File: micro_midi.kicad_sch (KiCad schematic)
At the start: 67 parts, among them U1 74HC595, U2 Arduino_Micro, U3 74HC595

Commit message: resistor change and pdf
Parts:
- R1, R10, R11, R12, R13, R14, R15, R16, R2, R3, R4, R5, R6, R7, R8, R9: footprint ScottoKeebs_Components:Resistor_0402 -> Resistor_THT:R_Axial_DIN0204_L3.6mm_D1.6mm_P1.90mm_Vertical
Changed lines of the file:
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@@
 			)
 		)
-		(property "Footprint" "ScottoKeebs_Components:Resistor_0402"
+		(property "Footprint" "Resistor_THT:R_Axial_DIN0204_L3.6mm_D1.6mm_P1.90mm_Vertical"
 			(at 218.44 124.968 0)
 			(effects
@@
 			)
 		)
-		(property "Footprint" "ScottoKeebs_Components:Resistor_0402"
+		(property "Footprint" "Resistor_THT:R_Axial_DIN0204_L3.6mm_D1.6mm_P1.90mm_Vertical"
 			(at 218.44 114.808 0)
 			(effects
@@
 			)
 		)
-		(property "Footprint" "ScottoKeebs_Components:Resistor_0402"
+		(property "Footprint" "Resistor_THT:R_Axial_DIN0204_L3.6mm_D1.6mm_P1.90mm_Vertical"
 			(at 218.44 112.268 0)
 			(effects
@@
 			)
 		)
-		(property "Footprint" "ScottoKeebs_Components:Resistor_0402"
+		(property "Footprint" "Resistor_THT:R_Axial_DIN0204_L3.6mm_D1.6mm_P1.90mm_Vertical"
 			(at 218.44 117.348 0)
 			(effects
@@
 			)
 		)
-		(property "Footprint" "ScottoKeebs_Components:Resistor_0402"
+		(property "Footprint" "Resistor_THT:R_Axial_DIN0204_L3.6mm_D1.6mm_P1.90mm_Vertical"
 			(at 218.44 66.548 0)
 			(effects
@@
 			)
 		)
-		(property "Footprint" "ScottoKeebs_Components:Resistor_0402"
+		(property "Footprint" "Resistor_THT:R_Axial_DIN0204_L3.6mm_D1.6mm_P1.90mm_Vertical"
 			(at 218.44 71.628 0)
 			(effects
@@
 			)
 		)
-		(property "Footprint" "ScottoKeebs_Components:Resistor_0402"
+		(property "Footprint" "Resistor_THT:R_Axial_DIN0204_L3.6mm_D1.6mm_P1.90mm_Vertical"
 			(at 218.44 109.728 0)
 			(effects
@@
 			)
 		)
-		(property "Footprint" "ScottoKeebs_Components:Resistor_0402"
+		(property "Footprint" "Resistor_THT:R_Axial_DIN0204_L3.6mm_D1.6mm_P1.90mm_Vertical"
 			(at 218.44 58.928 0)
 			(effects
@@
 			)
 		)
-		(property "Footprint" "ScottoKeebs_Components:Resistor_0402"
+		(property "Footprint" "Resistor_THT:R_Axial_DIN0204_L3.6mm_D1.6mm_P1.90mm_Vertical"
 			(at 218.44 64.008 0)
 			(effects
@@
 			)
 		)
-		(property "Footprint" "ScottoKeebs_Components:Resistor_0402"
+		(property "Footprint" "Resistor_THT:R_Axial_DIN0204_L3.6mm_D1.6mm_P1.90mm_Vertical"
 			(at 218.44 107.188 0)
 			(effects
@@
 			)
 		)
-		(property "Footprint" "ScottoKeebs_Components:Resistor_0402"
+		(property "Footprint" "Resistor_THT:R_Axial_DIN0204_L3.6mm_D1.6mm_P1.90mm_Vertical"
 			(at 218.44 61.468 0)
 			(effects
@@
 			)
 		)
-		(property "Footprint" "ScottoKeebs_Components:Resistor_0402"
+		(property "Footprint" "Resistor_THT:R_Axial_DIN0204_L3.6mm_D1.6mm_P1.90mm_Vertical"
 			(at 218.44 122.428 0)
 			(effects
@@
 			)
 		)
-		(property "Footprint" "ScottoKeebs_Components:Resistor_0402"
+		(property "Footprint" "Resistor_THT:R_Axial_DIN0204_L3.6mm_D1.6mm_P1.90mm_Vertical"
 			(at 218.44 69.088 0)
 			(effects
@@
 			)
 		)
-		(property "Footprint" "ScottoKeebs_Components:Resistor_0402"
+		(property "Footprint" "Resistor_THT:R_Axial_DIN0204_L3.6mm_D1.6mm_P1.90mm_Vertical"
 			(at 218.44 56.388 0)
 			(effects
@@
 			)
 		)
-		(property "Footprint" "ScottoKeebs_Components:Resistor_0402"
+		(property "Footprint" "Resistor_THT:R_Axial_DIN0204_L3.6mm_D1.6mm_P1.90mm_Vertical"
 			(at 218.44 119.888 0)
 			(effects
@@
 			)
 		)
-		(property "Footprint" "ScottoKeebs_Components:Resistor_0402"
+		(property "Footprint" "Resistor_THT:R_Axial_DIN0204_L3.6mm_D1.6mm_P1.90mm_Vertical"
 			(at 218.44 74.168 0)
 			(effects

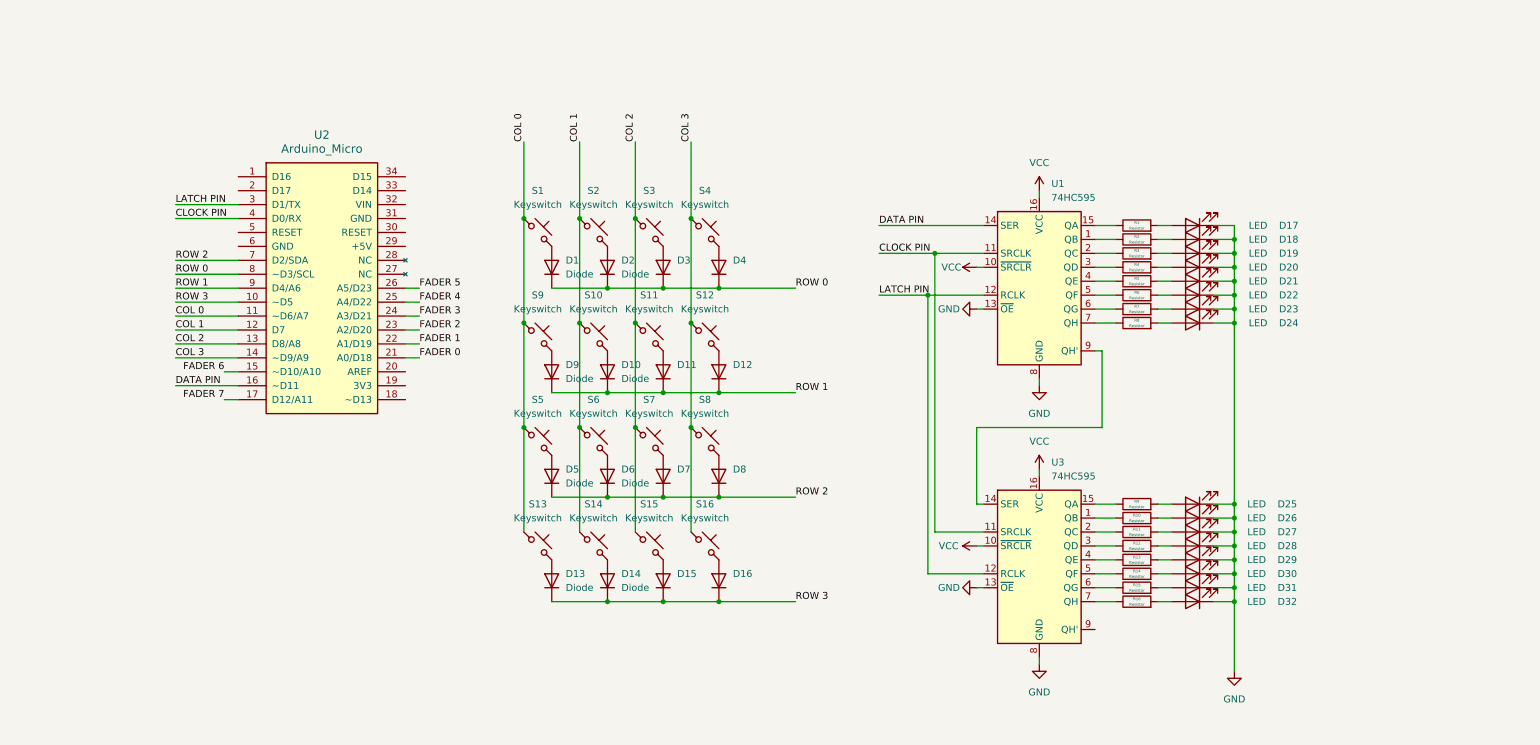
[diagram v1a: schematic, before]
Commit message: nearing completion
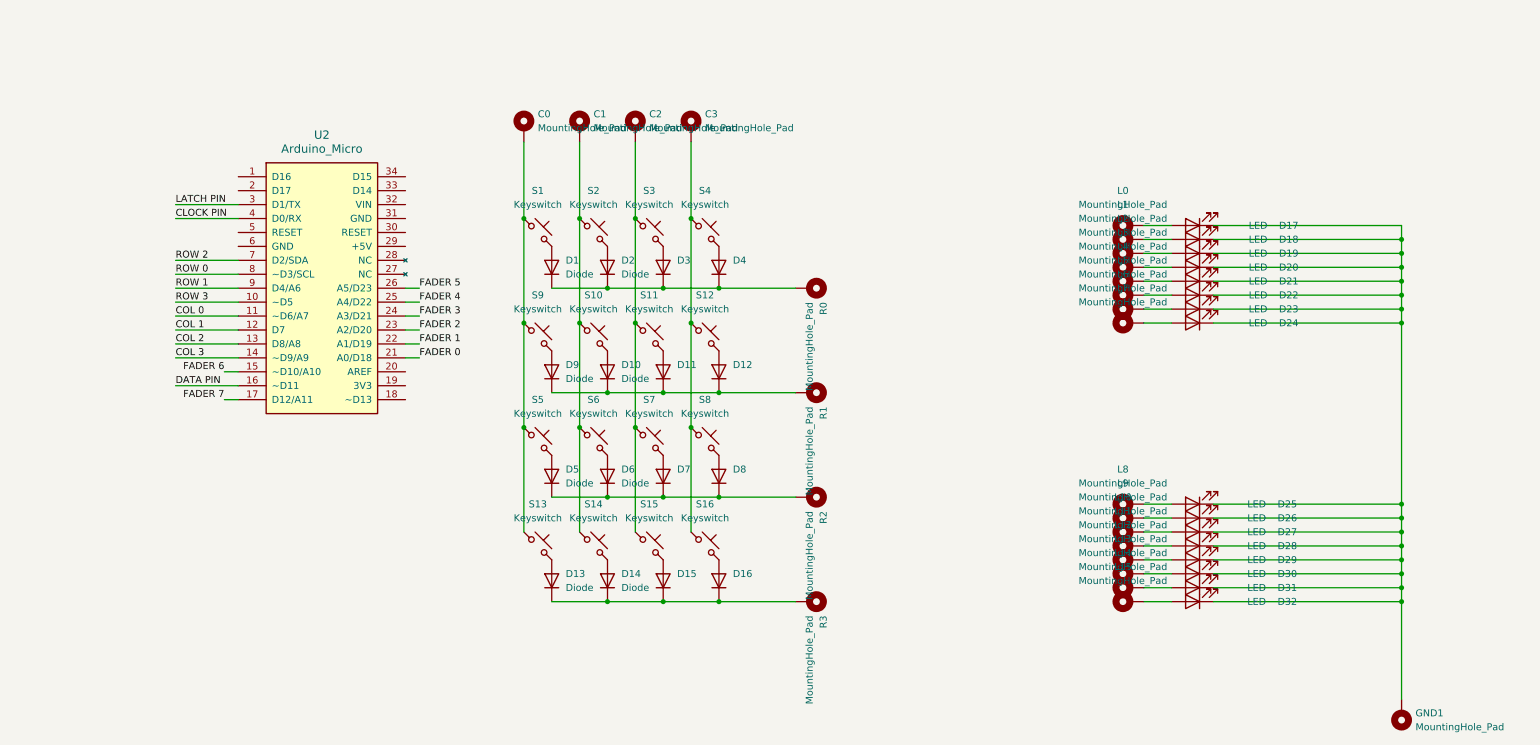
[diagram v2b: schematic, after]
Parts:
- removed R1, R10, R11, R12, R13, R14, R15, R16, R2, R3, R4, R5, R6, R7, R8, R9: Resistor, Resistor_THT:R_Axial_DIN0204_L3.6mm_D1.6mm_P1.90mm_Vertical, symbol ScottoKeebs:Placeholder_Resistor
- removed U1, U3: 74HC595, Package_SO:SSOP-16_5.3x6.2mm_P0.65mm, symbol 74xx:74HC595
- added C0, C1, C2, C3, GND1, L0, L1, L10, L11, L12, L13, L14, L15, L2, L3, L4, L5, L6, L7, L8, L9, R0, R1, R2, R3: MountingHole_Pad, TestPoint:TestPoint_Plated_Hole_D3.0mm, symbol Mechanical:MountingHole_Pad
- U2: footprint Arduino:Arduino_Micro -> (none)
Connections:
- net COL 0: no longer S1.1, S13.1, S5.1, S9.1
- net COL 1: no longer S10.1, S14.1, S2.1, S6.1
- net COL 2: no longer S11.1, S15.1, S3.1, S7.1
- net COL 3: no longer S12.1, S16.1, S4.1, S8.1
- net ROW 0: no longer D1.1 (K), D2.1 (K), D3.1 (K), D4.1 (K)
- net ROW 1: no longer D10.1 (K), D11.1 (K), D12.1 (K), D9.1 (K)
- net ROW 2: no longer D5.1 (K), D6.1 (K), D7.1 (K), D8.1 (K)
- net ROW 3: no longer D13.1 (K), D14.1 (K), D15.1 (K), D16.1 (K)
- net at D24.2 (A): now also L7.1
- net at D32.2 (A): now also L15.1
- net at D31.2 (A): now also L14.1
- net at D26.2 (A): now also L9.1
- net at D23.2 (A): now also L6.1
- net at D22.2 (A): now also L5.1
- net at D28.2 (A): now also L11.1
- net at D27.2 (A): now also L10.1
- net at D29.2 (A): now also L12.1
- net at D21.2 (A): now also L4.1
- net at D25.2 (A): now also L8.1
- net at D17.2 (A): now also L0.1
- net at D18.2 (A): now also L1.1
- net at D30.2 (A): now also L13.1
- net at D20.2 (A): now also L3.1
- net at D19.2 (A): now also L2.1
- net GND: no longer names the net of D17.1 (K), D18.1 (K), D19.1 (K), D20.1 (K), D21.1 (K), D22.1 (K), D23.1 (K), D24.1 (K), D25.1 (K), D26.1 (K), D27.1 (K), D28.1 (K), D29.1 (K), D30.1 (K), D31.1 (K), D32.1 (K)
- net GND: now also GND1.1
- new net: D10.1 (K), D11.1 (K), D12.1 (K), D9.1 (K), R1.1
- new net: C1.1, S10.1, S14.1, S2.1, S6.1
- new net: D13.1 (K), D14.1 (K), D15.1 (K), D16.1 (K), R3.1
- new net: D5.1 (K), D6.1 (K), D7.1 (K), D8.1 (K), R2.1
- new net: D1.1 (K), D2.1 (K), D3.1 (K), D4.1 (K), R0.1
- new net: C3.1, S12.1, S16.1, S4.1, S8.1
- new net: C0.1, S1.1, S13.1, S5.1, S9.1
- new net: C2.1, S11.1, S15.1, S3.1, S7.1

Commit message: updates
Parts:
- C0, C1, C2, C3, GND1, L0, L1, L10, L11, L12, L13, L14, L15, L2, L3, L4, L5, L6, L7, L8, L9, R0, R1, R2, R3: footprint TestPoint:TestPoint_Plated_Hole_D3.0mm -> CustomLib:THROUGH HOLE PAD 1.7MM HOLE 3.0MM PAD
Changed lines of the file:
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@@
 			)
 		)
-		(property "Footprint" "TestPoint:TestPoint_Plated_Hole_D3.0mm"
+		(property "Footprint" "CustomLib:THROUGH HOLE PAD 1.7MM HOLE 3.0MM PAD"
 			(at 158.75 85.09 0)
 			(effects
@@
 			)
 		)
-		(property "Footprint" "TestPoint:TestPoint_Plated_Hole_D3.0mm"
+		(property "Footprint" "CustomLib:THROUGH HOLE PAD 1.7MM HOLE 3.0MM PAD"
 			(at 116.84 36.83 0)
 			(effects
@@
 			)
 		)
-		(property "Footprint" "TestPoint:TestPoint_Plated_Hole_D3.0mm"
+		(property "Footprint" "CustomLib:THROUGH HOLE PAD 1.7MM HOLE 3.0MM PAD"
 			(at 217.17 120.65 0)
 			(effects
@@
 			)
 		)
-		(property "Footprint" "TestPoint:TestPoint_Plated_Hole_D3.0mm"
+		(property "Footprint" "CustomLib:THROUGH HOLE PAD 1.7MM HOLE 3.0MM PAD"
 			(at 266.7 143.51 0)
 			(effects
@@
 			)
 		)
-		(property "Footprint" "TestPoint:TestPoint_Plated_Hole_D3.0mm"
+		(property "Footprint" "CustomLib:THROUGH HOLE PAD 1.7MM HOLE 3.0MM PAD"
 			(at 217.17 113.03 0)
 			(effects
@@
 			)
 		)
-		(property "Footprint" "TestPoint:TestPoint_Plated_Hole_D3.0mm"
+		(property "Footprint" "CustomLib:THROUGH HOLE PAD 1.7MM HOLE 3.0MM PAD"
 			(at 217.17 107.95 0)
 			(effects
@@
 			)
 		)
-		(property "Footprint" "TestPoint:TestPoint_Plated_Hole_D3.0mm"
+		(property "Footprint" "CustomLib:THROUGH HOLE PAD 1.7MM HOLE 3.0MM PAD"
 			(at 217.17 57.15 0)
 			(effects
@@
 			)
 		)
-		(property "Footprint" "TestPoint:TestPoint_Plated_Hole_D3.0mm"
+		(property "Footprint" "CustomLib:THROUGH HOLE PAD 1.7MM HOLE 3.0MM PAD"
 			(at 106.68 36.83 0)
 			(effects
@@
 			)
 		)
-		(property "Footprint" "TestPoint:TestPoint_Plated_Hole_D3.0mm"
+		(property "Footprint" "CustomLib:THROUGH HOLE PAD 1.7MM HOLE 3.0MM PAD"
 			(at 217.17 59.69 0)
 			(effects
@@
 			)
 		)
-		(property "Footprint" "TestPoint:TestPoint_Plated_Hole_D3.0mm"
+		(property "Footprint" "CustomLib:THROUGH HOLE PAD 1.7MM HOLE 3.0MM PAD"
 			(at 217.17 105.41 0)
 			(effects
@@
 			)
 		)
-		(property "Footprint" "TestPoint:TestPoint_Plated_Hole_D3.0mm"
+		(property "Footprint" "CustomLib:THROUGH HOLE PAD 1.7MM HOLE 3.0MM PAD"
 			(at 217.17 123.19 0)
 			(effects
@@
 			)
 		)
-		(property "Footprint" "TestPoint:TestPoint_Plated_Hole_D3.0mm"
+		(property "Footprint" "CustomLib:THROUGH HOLE PAD 1.7MM HOLE 3.0MM PAD"
 			(at 217.17 64.77 0)
 			(effects
@@
 			)
 		)
-		(property "Footprint" "TestPoint:TestPoint_Plated_Hole_D3.0mm"
+		(property "Footprint" "CustomLib:THROUGH HOLE PAD 1.7MM HOLE 3.0MM PAD"
 			(at 217.17 72.39 0)
 			(effects
@@
 			)
 		)
-		(property "Footprint" "TestPoint:TestPoint_Plated_Hole_D3.0mm"
+		(property "Footprint" "CustomLib:THROUGH HOLE PAD 1.7MM HOLE 3.0MM PAD"
 			(at 217.17 69.85 0)
 			(effects
@@
 			)
 		)
-		(property "Footprint" "TestPoint:TestPoint_Plated_Hole_D3.0mm"
+		(property "Footprint" "CustomLib:THROUGH HOLE PAD 1.7MM HOLE 3.0MM PAD"
 			(at 137.16 36.83 0)
 			(effects
@@
 			)
 		)
-		(property "Footprint" "TestPoint:TestPoint_Plated_Hole_D3.0mm"
+		(property "Footprint" "CustomLib:THROUGH HOLE PAD 1.7MM HOLE 3.0MM PAD"
 			(at 158.75 66.04 0)
 			(effects
@@
 			)
 		)
-		(property "Footprint" "TestPoint:TestPoint_Plated_Hole_D3.0mm"
+		(property "Footprint" "CustomLib:THROUGH HOLE PAD 1.7MM HOLE 3.0MM PAD"
 			(at 217.17 62.23 0)
 			(effects
@@
 			)
 		)
-		(property "Footprint" "TestPoint:TestPoint_Plated_Hole_D3.0mm"
+		(property "Footprint" "CustomLib:THROUGH HOLE PAD 1.7MM HOLE 3.0MM PAD"
 			(at 217.17 118.11 0)
 			(effects
@@
 			)
 		)
-		(property "Footprint" "TestPoint:TestPoint_Plated_Hole_D3.0mm"
+		(property "Footprint" "CustomLib:THROUGH HOLE PAD 1.7MM HOLE 3.0MM PAD"
 			(at 217.17 115.57 0)
 			(effects
@@
 			)
 		)
-		(property "Footprint" "TestPoint:TestPoint_Plated_Hole_D3.0mm"
+		(property "Footprint" "CustomLib:THROUGH HOLE PAD 1.7MM HOLE 3.0MM PAD"
 			(at 158.75 123.19 0)
 			(effects
@@
 			)
 		)
-		(property "Footprint" "TestPoint:TestPoint_Plated_Hole_D3.0mm"
+		(property "Footprint" "CustomLib:THROUGH HOLE PAD 1.7MM HOLE 3.0MM PAD"
 			(at 127 36.83 0)
 			(effects
@@
 			)
 		)
-		(property "Footprint" "TestPoint:TestPoint_Plated_Hole_D3.0mm"
+		(property "Footprint" "CustomLib:THROUGH HOLE PAD 1.7MM HOLE 3.0MM PAD"
 			(at 158.75 104.14 0)
 			(effects
@@
 			)
 		)
-		(property "Footprint" "TestPoint:TestPoint_Plated_Hole_D3.0mm"
+		(property "Footprint" "CustomLib:THROUGH HOLE PAD 1.7MM HOLE 3.0MM PAD"
 			(at 217.17 54.61 0)
 			(effects
@@
 			)
 		)
-		(property "Footprint" "TestPoint:TestPoint_Plated_Hole_D3.0mm"
+		(property "Footprint" "CustomLib:THROUGH HOLE PAD 1.7MM HOLE 3.0MM PAD"
 			(at 217.17 110.49 0)
 			(effects
@@
 			)
 		)
-		(property "Footprint" "TestPoint:TestPoint_Plated_Hole_D3.0mm"
+		(property "Footprint" "CustomLib:THROUGH HOLE PAD 1.7MM HOLE 3.0MM PAD"
 			(at 217.17 67.31 0)
 			(effects

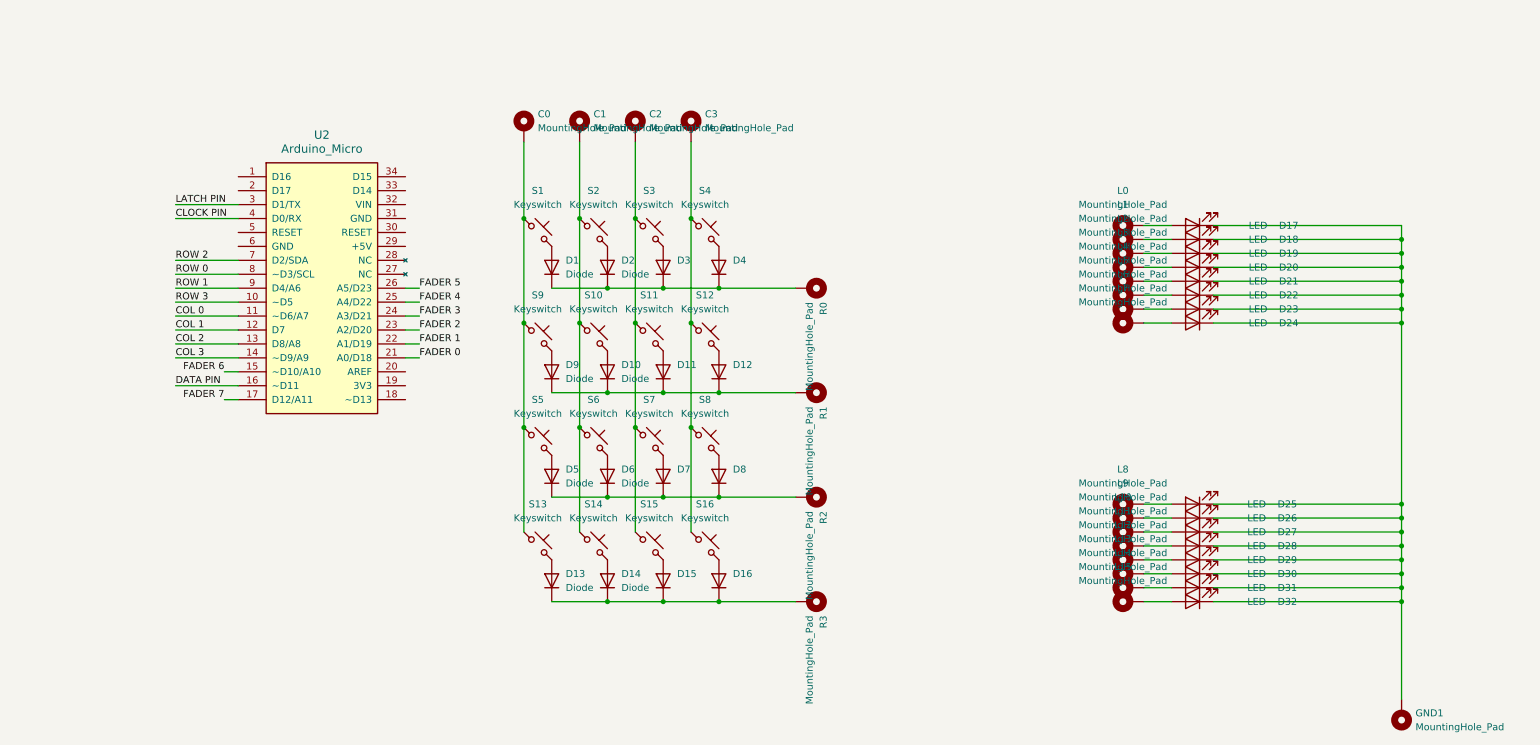
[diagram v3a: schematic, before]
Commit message: cleaned repo and readme
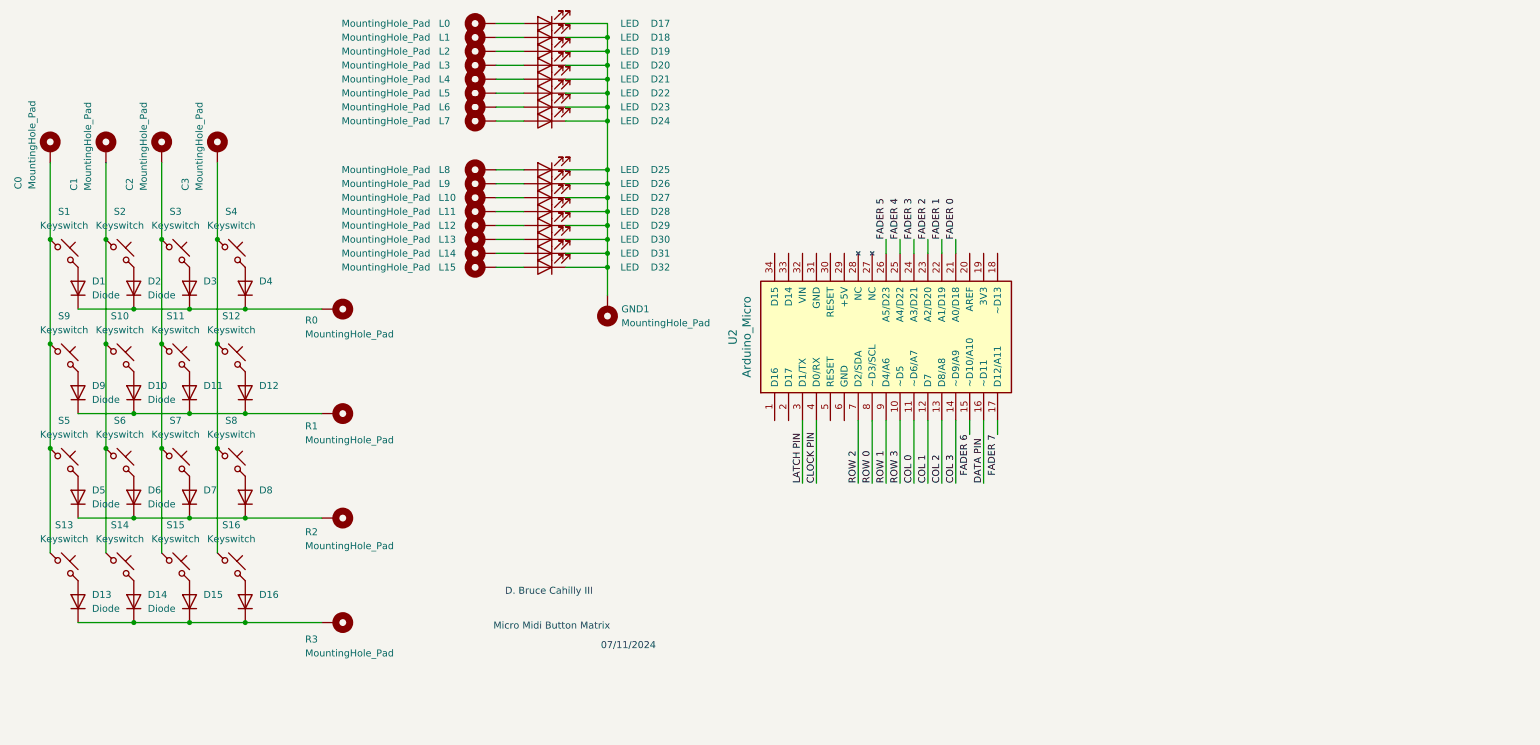
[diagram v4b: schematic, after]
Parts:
- U2: now left out of the parts list
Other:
- note added: "07/11/2024"
- note added: "D. Bruce Cahilly III"
- note added: "Micro Midi Button Matrix"
- moved on the sheet: C0, C1, C2, C3, D1, D10, D11, D12, D13, D14, D15, D16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
